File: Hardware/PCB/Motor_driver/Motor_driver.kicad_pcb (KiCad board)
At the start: 4 copper layers, 70 x 90 mm, 73 parts, among them IC1 A89307KETSR-J, IC2 STM32L412KBT6, J1 ENCODER, J2 USB_C, J3 PAD_MOTEUR, J4 Debug, J5 Conn_01x01_Pin, J6 Conn_01x01_Pin, J7 Conn_01x01_Pin, J8 Conn_01x01_Pin

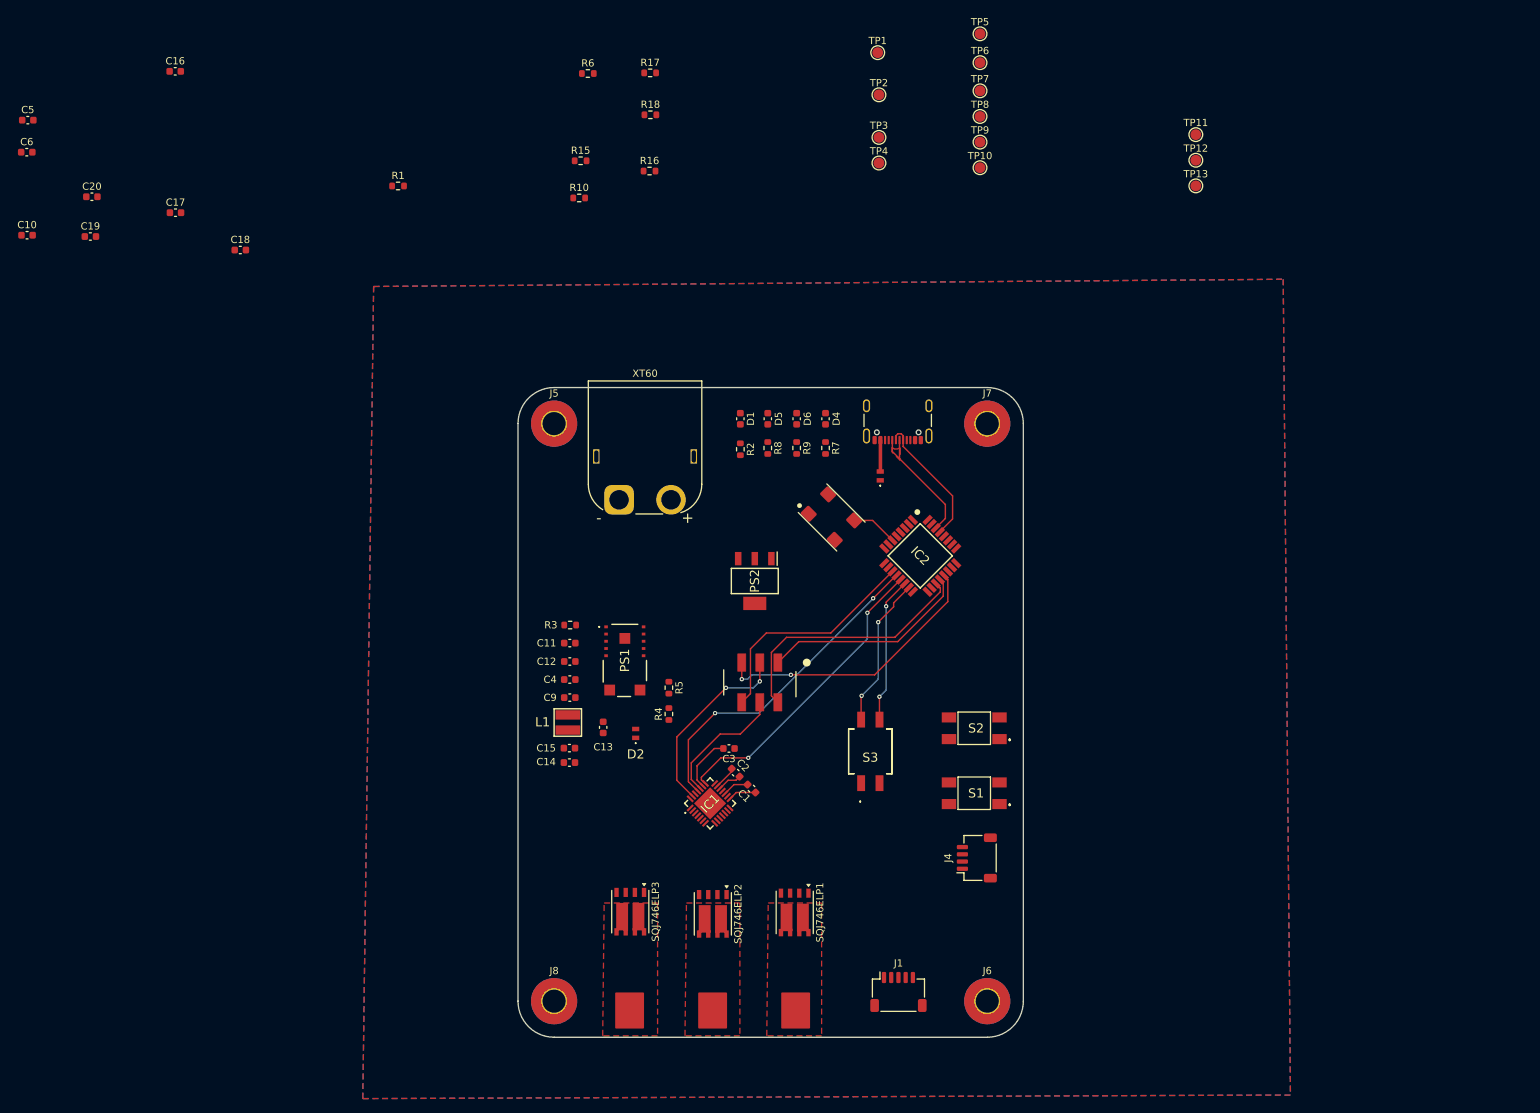
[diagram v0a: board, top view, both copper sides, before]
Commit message: update
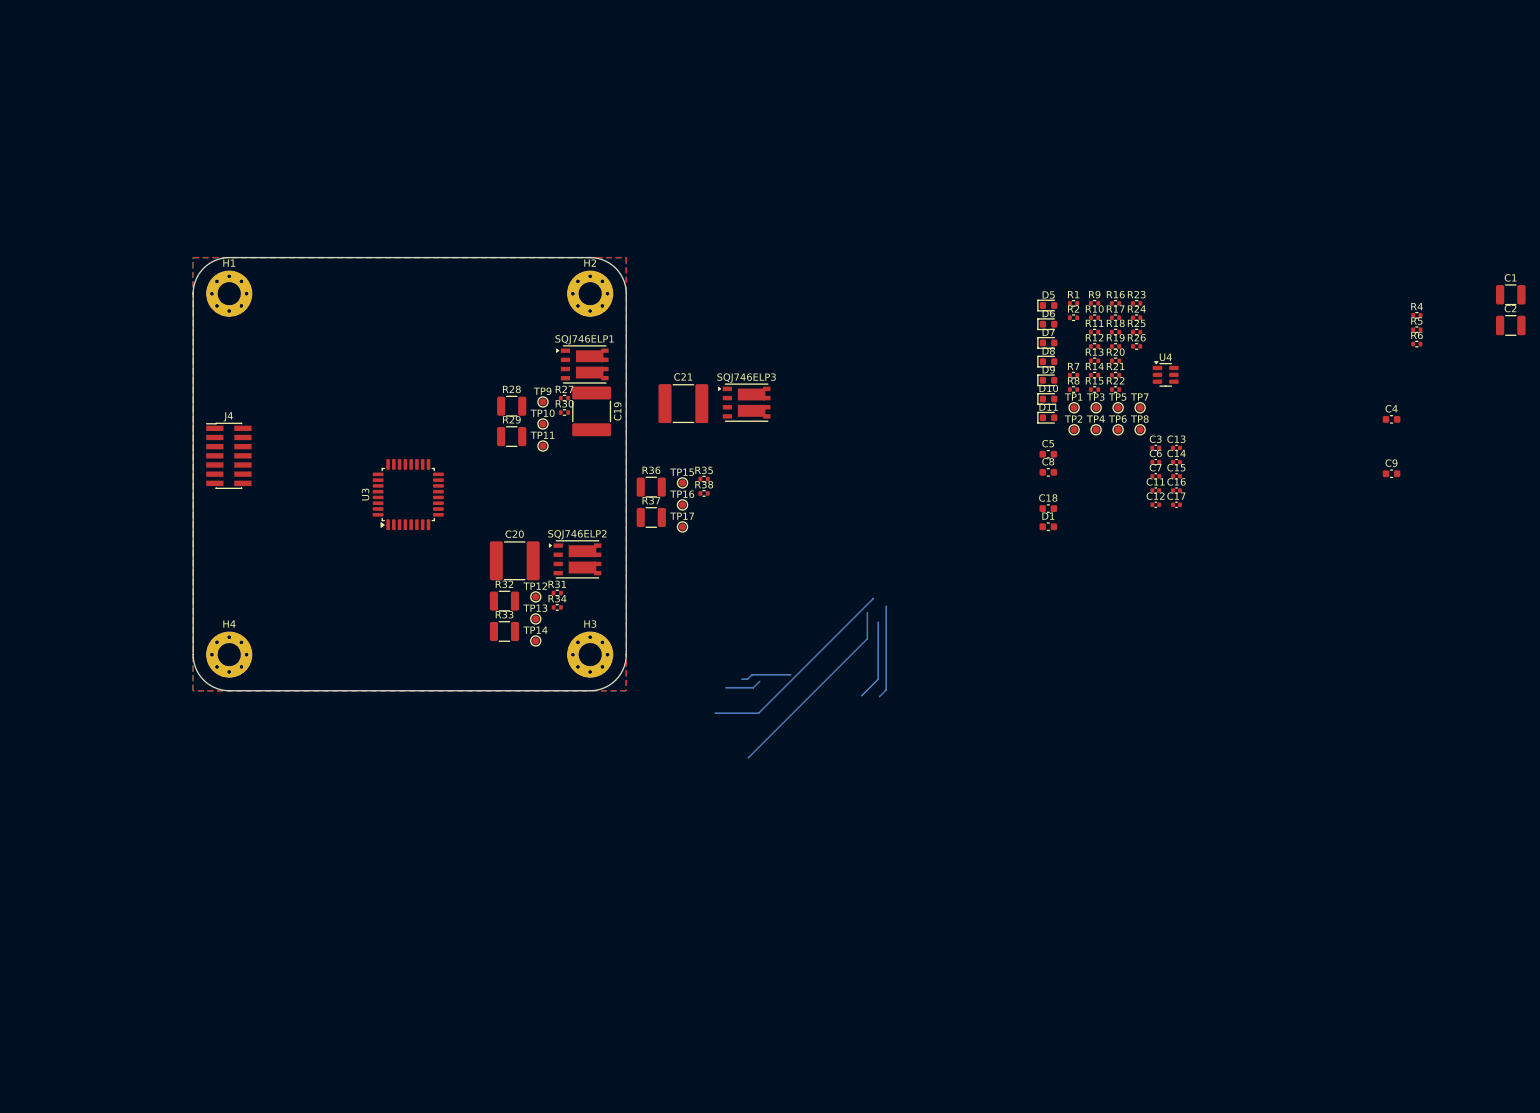
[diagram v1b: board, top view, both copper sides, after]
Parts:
- removed C10: 100n, Capacitor_SMD:C_0603_1608Metric
- removed D2: 824045817, SamacSys_Parts:824045817
- removed D4: LED, Capacitor_SMD:C_0603_1608Metric
- removed IC1: A89307KETSR-J, SamacSys_Parts:A8519KETTRR1
- removed IC2: STM32L412KBT6, SamacSys_Parts:QFP80P900X900X160-32N
- removed J1: ENCODER, Connector_JST:JST_SH_SM05B-SRSS-TB_1x05-1MP_P1.00mm_Horizontal
- removed J2: USB_C, Connector_USB:USB_C_Receptacle_GCT_USB4105-xx-A_16P_TopMnt_Horizontal
- removed J3: PAD_MOTEUR, Custom:Solder Pad x3
- removed J5, J6, J7, J8: Conn_01x01_Pin, MountingHole:MountingHole_3.2mm_M3_Pad_TopBottom
- removed L1: 10µH, SamacSys_Parts:WE-MAPI_3020
- removed Oscillator1: ~, Custom:Oscillator 7x5mm
- removed PS1: 171013801, SamacSys_Parts:171013801
- removed PS2: AZ1117CH2-3.3TRG1, SamacSys_Parts:SOT230P700X180-4N
- removed R3: 5.6k, Resistor_SMD:R_0603_1608Metric
- removed S1, S2: 430181038816, SamacSys_Parts:430181038816
- removed S3: 418121270802, SamacSys_Parts:418121270802
- removed U1: ~, Custom:452406020024
- removed XT60: PWR_CONN, Connector_AMASS:AMASS_XT60PW-M_1x02_P7.20mm_Horizontal
- added C21: 10u, Capacitor_SMD:C_2220_5750Metric, F.Cu at (112.9, 65.2)
- added C7: 220n, Capacitor_SMD:C_0402_1005Metric, F.Cu at (178.3, 75.3)
- added C8: 22u, Capacitor_SMD:C_0603_1608Metric, F.Cu at (163.5, 74.8)
- added D10: LED_0, LED_SMD:LED_0603_1608Metric, F.Cu at (163.5, 64.6)
- added D11: LED_1, LED_SMD:LED_0603_1608Metric, F.Cu at (163.5, 67.2)
- added D8: LED, LED_SMD:LED_0603_1608Metric, F.Cu at (163.5, 59.4)
- added D9: LED, LED_SMD:LED_0603_1608Metric, F.Cu at (163.5, 62.0)
- added H1: MountingHole_Pad, MountingHole:MountingHole_3.2mm_M3_Pad_Via, F.Cu at (50.0, 50.0)
- added H2: MountingHole_Pad, MountingHole:MountingHole_3.2mm_M3_Pad_Via, F.Cu at (100.0, 50.0)
- added H3: MountingHole_Pad, MountingHole:MountingHole_3.2mm_M3_Pad_Via, F.Cu at (100.0, 100.0)
- added H4: MountingHole_Pad, MountingHole:MountingHole_3.2mm_M3_Pad_Via, F.Cu at (50.0, 100.0)
- added R11: 1k5, Resistor_SMD:R_0402_1005Metric, F.Cu at (169.9, 55.3)
- added R12: 10k, Resistor_SMD:R_0402_1005Metric, F.Cu at (169.9, 57.3)
- added R13: 10k, Resistor_SMD:R_0402_1005Metric, F.Cu at (169.9, 59.3)
- added R14: 10k, Resistor_SMD:R_0402_1005Metric, F.Cu at (169.9, 61.3)
- added R19: 10k, Resistor_SMD:R_0402_1005Metric, F.Cu at (172.8, 57.3)
- added R20: 5k1, Resistor_SMD:R_0402_1005Metric, F.Cu at (172.8, 59.3)
- added R21: 5k1, Resistor_SMD:R_0402_1005Metric, F.Cu at (172.8, 61.3)
- added R22: 10k, Resistor_SMD:R_0402_1005Metric, F.Cu at (172.8, 63.3)
- added R23: 10k, Resistor_SMD:R_0402_1005Metric, F.Cu at (175.7, 51.3)
- added R24: 10k, Resistor_SMD:R_0402_1005Metric, F.Cu at (175.7, 53.3)
- added R25: 1k, Resistor_SMD:R_0402_1005Metric, F.Cu at (175.7, 55.3)
- added R26: 1k, Resistor_SMD:R_0402_1005Metric, F.Cu at (175.7, 57.3)
- added R27: 10k, Resistor_SMD:R_0402_1005Metric, F.Cu at (96.4, 64.5)
- added R28: 120, Resistor_SMD:R_1210_3225Metric, F.Cu at (89.1, 65.6)
- added R29: 120, Resistor_SMD:R_1210_3225Metric, F.Cu at (89.1, 69.8)
- added R30: 10k, Resistor_SMD:R_0402_1005Metric, F.Cu at (96.4, 66.5)
- added R31: 10k, Resistor_SMD:R_0402_1005Metric, F.Cu at (95.4, 91.5)
- added R32: 120, Resistor_SMD:R_1210_3225Metric, F.Cu at (88.1, 92.6)
- added R33: 120, Resistor_SMD:R_1210_3225Metric, F.Cu at (88.1, 96.8)
- added R34: 10k, Resistor_SMD:R_0402_1005Metric, F.Cu at (95.4, 93.5)
- added R35: 10k, Resistor_SMD:R_0402_1005Metric, F.Cu at (115.8, 75.7)
- added R36: 120, Resistor_SMD:R_1210_3225Metric, F.Cu at (108.5, 76.8)
- added R37: 120, Resistor_SMD:R_1210_3225Metric, F.Cu at (108.5, 81.0)
- added R38: 10k, Resistor_SMD:R_0402_1005Metric, F.Cu at (115.8, 77.7)
- added TP14: GATE C, TestPoint:TestPoint_Pad_D1.0mm, F.Cu at (92.5, 98.1)
- added TP15: GATE C, TestPoint:TestPoint_Pad_D1.0mm, F.Cu at (112.8, 76.2)
- added TP16: GATE C, TestPoint:TestPoint_Pad_D1.0mm, F.Cu at (112.8, 79.3)
- added TP17: GATE C, TestPoint:TestPoint_Pad_D1.0mm, F.Cu at (112.8, 82.3)
- added U3: STM32L412KBTx, Package_QFP:LQFP-32_7x7mm_P0.8mm, F.Cu at (74.8, 77.8)
- added U4: USBLC6-2SC6, Package_TO_SOT_SMD:SOT-23-6, F.Cu at (179.7, 61.2)
- C1, C2: value 22µF -> 4u7; footprint Capacitor_SMD:C_0603_1608Metric -> Capacitor_SMD:C_1210_3225Metric
- C11: value 1µF -> 10n; footprint Capacitor_SMD:C_0603_1608Metric -> Capacitor_SMD:C_0402_1005Metric
- C12, C15: value 4.7µF -> 100n; footprint Capacitor_SMD:C_0603_1608Metric -> Capacitor_SMD:C_0402_1005Metric
- C13: value 22µF -> 10n; footprint Capacitor_SMD:C_0603_1608Metric -> Capacitor_SMD:C_0402_1005Metric
- C14: value 4.7µF -> 10n; footprint Capacitor_SMD:C_0603_1608Metric -> Capacitor_SMD:C_0402_1005Metric
- C16, C17: value 100nF -> 100n; footprint Capacitor_SMD:C_0603_1608Metric -> Capacitor_SMD:C_0402_1005Metric
- C18: value 10µF -> 4u7
- C19: value 22µF -> 10u; footprint Capacitor_SMD:C_0603_1608Metric -> Capacitor_SMD:C_2220_5750Metric
- C20: value 15pF -> 10u; footprint Capacitor_SMD:C_0603_1608Metric -> Capacitor_SMD:C_2220_5750Metric
- C3: value 22µF -> 220n; footprint Capacitor_SMD:C_0603_1608Metric -> Capacitor_SMD:C_0402_1005Metric
- C4: value 4.7µF -> 1u
- C5: value 100n -> 10u
- C6: value 100n -> 220n; footprint Capacitor_SMD:C_0603_1608Metric -> Capacitor_SMD:C_0402_1005Metric
- C9: value 220µF -> 47u
- D5, D6: footprint Capacitor_SMD:C_0603_1608Metric -> LED_SMD:LED_0603_1608Metric
- D7: value 824045817 -> LED; footprint SamacSys_Parts:824045817 -> LED_SMD:LED_0603_1608Metric
- J4: value Debug -> Conn_ST_STDC14; footprint Connector_JST:JST_SH_SM04B-SRSS-TB_1x04-1MP_P1.00mm_Horizontal -> Connector_PinHeader_1.27mm:PinHeader_2x07_P1.27mm_Vertical_SMD
- R1: value 0.025 -> 1k7; footprint Resistor_SMD:R_0603_1608Metric -> Resistor_SMD:R_0402_1005Metric
- R10: value 10k -> 2k5; footprint Resistor_SMD:R_0603_1608Metric -> Resistor_SMD:R_0402_1005Metric
- R15, R16, R17, R18, R7, R8: footprint Resistor_SMD:R_0603_1608Metric -> Resistor_SMD:R_0402_1005Metric
- R2: value 200 -> 10k; footprint Resistor_SMD:R_0603_1608Metric -> Resistor_SMD:R_0402_1005Metric
- R4: value 402k -> 5k6; footprint Resistor_SMD:R_0603_1608Metric -> Resistor_SMD:R_0402_1005Metric
- R5: value 80k -> 402k; footprint Resistor_SMD:R_0603_1608Metric -> Resistor_SMD:R_0402_1005Metric
- R6: value 10k -> 80k6; footprint Resistor_SMD:R_0603_1608Metric -> Resistor_SMD:R_0402_1005Metric
- R9: value 1k5 -> 2k5; footprint Resistor_SMD:R_0603_1608Metric -> Resistor_SMD:R_0402_1005Metric
- TP1: value SDA -> 24V; footprint TestPoint:TestPoint_Pad_D1.5mm -> TestPoint:TestPoint_Pad_D1.0mm
- TP10: value BRAKE -> GATE C; footprint TestPoint:TestPoint_Pad_D1.5mm -> TestPoint:TestPoint_Pad_D1.0mm
- TP11: value 24V -> GATE C; footprint TestPoint:TestPoint_Pad_D1.5mm -> TestPoint:TestPoint_Pad_D1.0mm
- TP12: value 5V -> GATE C; footprint TestPoint:TestPoint_Pad_D1.5mm -> TestPoint:TestPoint_Pad_D1.0mm
- TP13: value 3.3V -> GATE C; footprint TestPoint:TestPoint_Pad_D1.5mm -> TestPoint:TestPoint_Pad_D1.0mm
- TP2: value SCL -> 5V_BUCK; footprint TestPoint:TestPoint_Pad_D1.5mm -> TestPoint:TestPoint_Pad_D1.0mm
- TP3: value RX -> 5V_USB; footprint TestPoint:TestPoint_Pad_D1.5mm -> TestPoint:TestPoint_Pad_D1.0mm
- TP4: value TX -> 5V; footprint TestPoint:TestPoint_Pad_D1.5mm -> TestPoint:TestPoint_Pad_D1.0mm
- TP5: value GATE C -> 3V3; footprint TestPoint:TestPoint_Pad_D1.5mm -> TestPoint:TestPoint_Pad_D1.0mm
- TP6: value GATE B -> PWM; footprint TestPoint:TestPoint_Pad_D1.5mm -> TestPoint:TestPoint_Pad_D1.0mm
- TP7: value GATE A -> DIR; footprint TestPoint:TestPoint_Pad_D1.5mm -> TestPoint:TestPoint_Pad_D1.0mm
- TP8: value PWM -> BRAKE; footprint TestPoint:TestPoint_Pad_D1.5mm -> TestPoint:TestPoint_Pad_D1.0mm
- TP9: value DIR -> GATE C; footprint TestPoint:TestPoint_Pad_D1.5mm -> TestPoint:TestPoint_Pad_D1.0mm
- moved C6 162.2 mm to (178.3, 73.3)
- moved C16 150.4 mm to (181.2, 77.3)
- moved C5 148.7 mm to (163.5, 72.2)
- moved C17 144.4 mm to (181.2, 79.2)
- moved C1 125.5 mm to (227.5, 50.1), turned to 0 degrees
- moved C2 124.0 mm to (227.5, 54.4), turned to 0 degrees
- moved R6 120.8 mm to (214.5, 57.0)
- moved C4 119.4 mm to (211.0, 67.4), turned to 0 degrees
- moved C9 118.0 mm to (211.0, 74.9), turned to 0 degrees
- moved J4 117.6 mm to (50.0, 72.5), turned to 0 degrees
- moved C18 117.5 mm to (163.5, 79.8)
- moved R4 117.4 mm to (214.5, 53.0), turned to 0 degrees
- moved R5 114.9 mm to (214.5, 55.0), turned to 0 degrees
- moved TP12 109.6 mm to (92.5, 92.0)
- moved TP13 109.4 mm to (92.5, 95.0)
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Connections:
- C1 pad 1: Net-(IC1-VCP) -> +24V
- C1 pad 2: +24V -> GND
- C11 pad 1: Net-(PS1-VCC) -> /BTN_1
- C12 pad 1: Net-(PS1-EN) -> GND
- C12 pad 2: GND -> /NRST
- C13 pad 1: Net-(D2-A) -> /BTN_2
- C14 pad 1: +24V -> /BTN_3
- C15 pad 1: +24V -> GND
- C15 pad 2: GND -> +3.3V
- C16 pad 1: Net-(IC2-PA15) -> +3.3V
- C17 pad 1: Net-(IC2-NRST) -> +3.3V
- C18 pad 1: +5V -> +3.3V
- C19 pad 1: +3.3V -> +24V
- C2 pad 1: Net-(IC1-CP1) -> +24V
- C2 pad 2: Net-(IC1-CP2) -> GND
- C20 pad 1: Net-(IC2-PA0-CK_IN) -> +24V
- C4 pad 1: Net-(PS1-EN) -> Net-(PS1-VCC)
- C5 pad 1: +3.3V -> +5V
- C6 pad 1: +3.3V -> Net-(IC1-CP1)
- C6 pad 2: GND -> Net-(IC1-CP2)
- C9 pad 1: Net-(PS1-EN) -> /5V_BUCK
- D1 pad 1: GND -> Net-(D1-K)
- D5 pad 2: +5V -> +24V
- D6 pad 2: +3.3V -> /5V_BUCK
- D7 pad 1: +5V -> Net-(D7-K)
- D7 pad 2: Net-(D7-A) -> /5V_USB
- J4 pad 1: SWCLK -> unconnected-(J4-NC-Pad1)
- J4 pad 2: SWDIO -> unconnected-(J4-NC-Pad2)
- J4 pad 3: SWO -> +3.3V
- J4 pad 4: GND -> /SWDIO
- R1 pad 1: GND -> Net-(D1-A)
- R1 pad 2: LSS -> +3.3V
- R10 pad 2: Net-(IC2-PA15) -> GND
- R15 pad 1: SDA -> /ADD_SEL_0
- R16 pad 1: SCL -> /BTN_2
- R16 pad 2: +3.3V -> Net-(R16-Pad2)
- R17 pad 1: +3.3V -> Net-(R16-Pad2)
- R17 pad 2: Net-(R17-Pad2) -> +3.3V
- R18 pad 1: +3.3V -> /BTN_3
- R2 pad 1: Net-(D1-A) -> Net-(D1-K)
- R2 pad 2: Net-(IC1-FAULT) -> +3.3V
- R4 pad 1: Net-(D2-A) -> Net-(PS1-FSW)
- R4 pad 2: Net-(PS1-FB) -> GND
- R5 pad 1: Net-(PS1-FB) -> /5V_BUCK
- R5 pad 2: GND -> Net-(PS1-FB)
- R6 pad 1: Net-(S1-CM) -> Net-(PS1-FB)
- R6 pad 2: Net-(IC2-NRST) -> GND
- R7 pad 1: Net-(D4-K) -> Net-(D5-K)
- R8 pad 1: Net-(D5-K) -> Net-(D6-K)
- R9 pad 1: Net-(D6-K) -> Net-(D7-K)
- SQJ746ELP1 pad 1: +24V -> /arm_bridge_A/Sx
- SQJ746ELP1 pad 2: Net-(IC1-GHC) -> Net-(SQJ746ELP1-G1)
- SQJ746ELP1 pad 3: LSS -> /LSS
- SQJ746ELP1 pad 4: GLC -> Net-(SQJ746ELP1-G2)
- SQJ746ELP1 pad 5: SC -> /arm_bridge_A/Sx
- SQJ746ELP1 pad 6: SC -> +24V
- SQJ746ELP2 pad 1: +24V -> /arm_bridge_B/Sx
- SQJ746ELP2 pad 2: Net-(IC1-GHB) -> Net-(SQJ746ELP2-G1)
- SQJ746ELP2 pad 3: LSS -> /LSS
- SQJ746ELP2 pad 4: GLB -> Net-(SQJ746ELP2-G2)
- SQJ746ELP2 pad 5: SB -> /arm_bridge_B/Sx
- SQJ746ELP2 pad 6: SB -> +24V
- SQJ746ELP3 pad 1: +24V -> /arm_bridge_C/Sx
- SQJ746ELP3 pad 2: Net-(IC1-GHA) -> Net-(SQJ746ELP3-G1)
- SQJ746ELP3 pad 3: LSS -> /LSS
- SQJ746ELP3 pad 4: GLA -> Net-(SQJ746ELP3-G2)
- SQJ746ELP3 pad 5: SA -> /arm_bridge_C/Sx
- SQJ746ELP3 pad 6: SA -> +24V
- TP1 pad 1: SDA -> +24V
- TP10 pad 1: BRAKE -> /arm_bridge_A/Sx
- TP11 pad 1: +24V -> /GLC
- TP12 pad 1: +5V -> /arm_bridge_B/GHx
- TP13 pad 1: +3.3V -> /arm_bridge_B/Sx
- TP2 pad 1: SCL -> /5V_BUCK
- TP3 pad 1: RX -> /5V_USB
- TP4 pad 1: TX -> +5V
- TP5 pad 1: Net-(IC1-GHC) -> +3.3V
- TP6 pad 1: Net-(IC1-GHB) -> /PWM_TIM1_CH1
- TP7 pad 1: Net-(IC1-GHA) -> DIR
- TP8 pad 1: PWM -> BRAKE
- TP9 pad 1: DIR -> /arm_bridge_A/GHx
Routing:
- net PA11: track 39.0 -> 0.00 mm, vias 2 -> 0
- net (no net): track 0.00 -> 36.2 mm
- net SCL: track 35.6 -> 0.00 mm
- net PWM: track 32.0 -> 0.00 mm
- net SDA: track 29.2 -> 0.00 mm
- net FG: track 26.4 -> 0.00 mm, vias 2 -> 0
- net Net-(IC2-PB1): track 21.0 -> 0.00 mm, vias 2 -> 0
- net Net-(IC2-PB0): track 20.3 -> 0.00 mm, vias 2 -> 0
- net TX: track 19.4 -> 0.00 mm
- net RX: track 18.4 -> 0.00 mm
- net SPD: track 18.1 -> 0.00 mm
- net DIR: track 46.0 -> 28.5 mm, vias 2 -> 0
- net BRAKE: track 42.0 -> 26.9 mm, vias 2 -> 0
- net Net-(IC1-VREG): track 7.78 -> 0.00 mm
- net Net-(IC2-PA0-CK_IN): track 6.45 -> 0.00 mm
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- added copper zone on In2.Cu, net +3.3V
- added copper zone on In2.Cu, net +5V
- removed copper zone on In2.Cu, net GND
- removed copper zone on F.Cu, net RX
- removed copper zone on F.Cu, net SA
- removed copper zone on F.Cu, net SB
- removed copper zone on F.Cu, net SC
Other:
- board size 70 x 90 mm -> 60 x 60 mm
